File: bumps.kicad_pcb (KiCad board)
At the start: 2 copper layers, 111.1 x 65.4 mm, 135 parts, among them M1 CONN_1, M2 CONN_1, M3 CONN_1, P1 DIL6, P10 Mot-A, P11 Mot-A, P12 Mot-X, P13 T1, P14 T2, P15 T3, P16 MPower, P17 PWM-2, P18 PWM-1, P19 END-X, P2 DIL6, P20 END-Y, P21 END-Z, P22 Mot-X, P23 Mot-Y, P24 Mot-Y, P25 Mot-Z, P26 Mot-Z, P27 Aux, P28 KillSwitch, P29 PWM, P3 Mot-E, P30 CONN_01X01, P31 CONN_01X01, P4 Mot-E, P5 DIL6, P6 DIL6, P7 DIL6, P8 P8 Header, P9 P9 Header, Q1 IRLB8743PBF, Q2 IRLB8743PBF, Q3 FDS9926A, Q4 FDS9926A, U1 Motor-2, U2 Motor-4, U3 Motor-5, U4 Motor-3, U5 Motor-1, U6 MC34063, U7 AP1117/3.3, U8 Opto

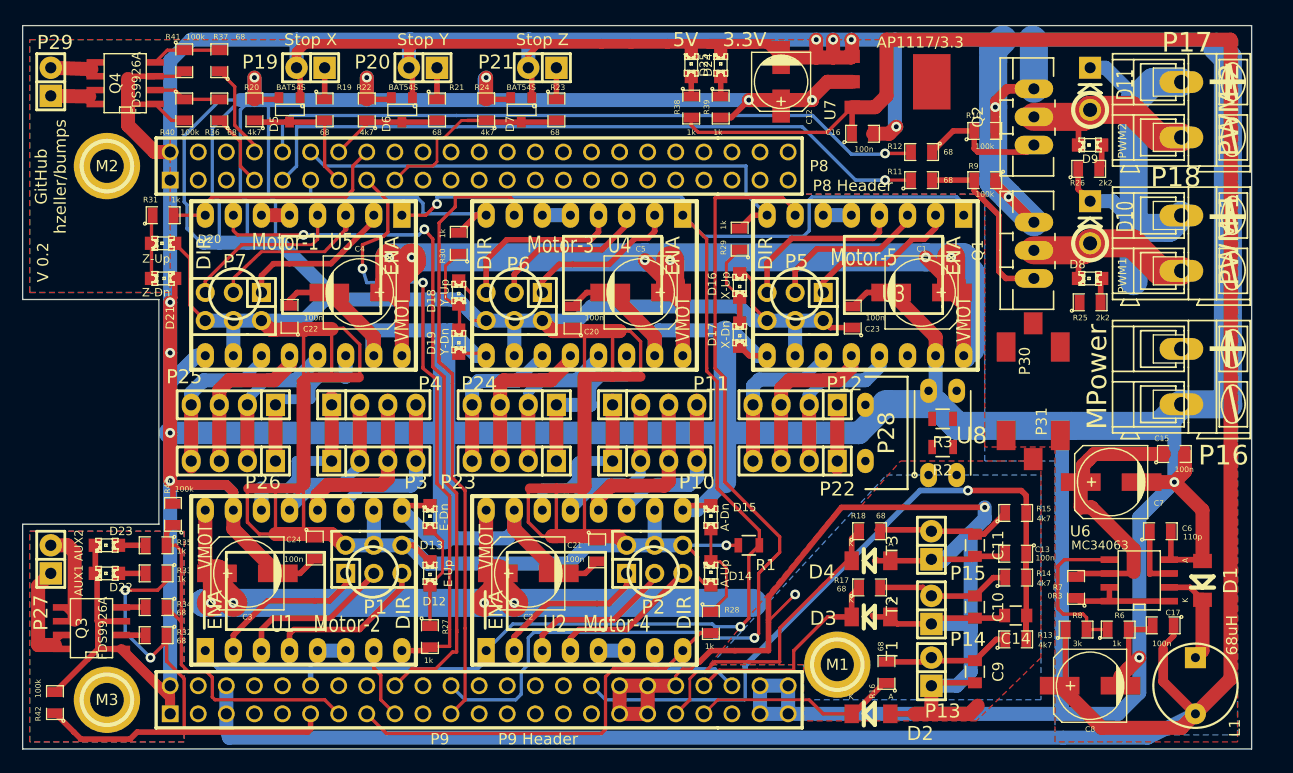
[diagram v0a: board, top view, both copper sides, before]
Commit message: o intermediate state.
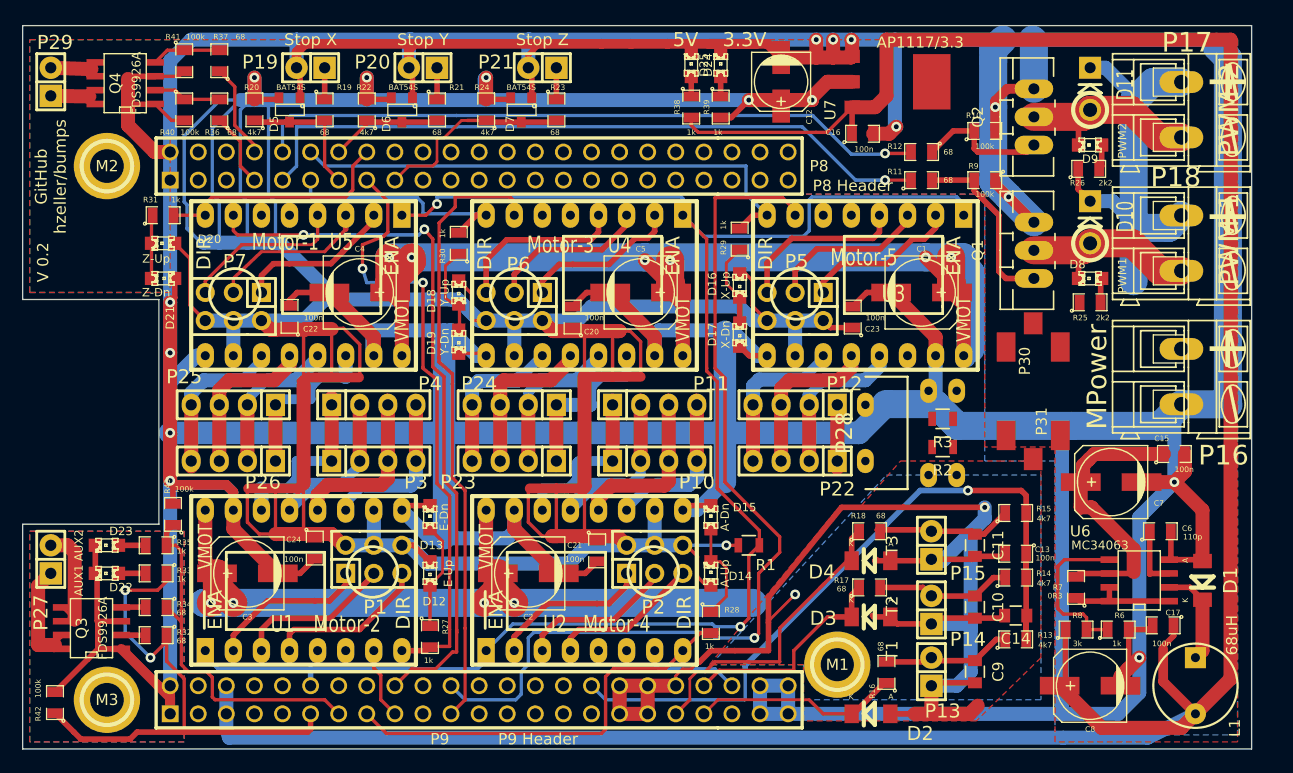
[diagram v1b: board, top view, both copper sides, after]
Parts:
- U8: moved to B.Cu
- turned P28 to 0 degrees
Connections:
- M1 pad 1: Net-(M1-Pad1) -> (no net)
- M2 pad 1: Net-(M2-Pad1) -> (no net)
- M3 pad 1: Net-(M3-Pad1) -> (no net)
- P8 pad 18: Net-(P8-Pad18) -> (no net)
- P8 pad 19: Net-(P8-Pad19) -> (no net)
- P8 pad 20: Net-(P8-Pad20) -> (no net)
- P8 pad 21: Net-(P8-Pad21) -> (no net)
- P8 pad 22: Net-(P8-Pad22) -> (no net)
- P8 pad 23: Net-(P8-Pad23) -> (no net)
- P8 pad 24: Net-(P8-Pad24) -> (no net)
- P8 pad 25: Net-(P8-Pad25) -> (no net)
- P8 pad 26: Net-(P8-Pad26) -> (no net)
- P8 pad 27: Net-(P8-Pad27) -> (no net)
- P8 pad 28: Net-(P8-Pad28) -> (no net)
- P8 pad 29: Net-(P8-Pad29) -> (no net)
- P8 pad 3: Net-(P8-Pad3) -> (no net)
- P8 pad 30: Net-(P8-Pad30) -> (no net)
- P8 pad 31: Net-(P8-Pad31) -> (no net)
- P8 pad 32: Net-(P8-Pad32) -> (no net)
- P8 pad 33: Net-(P8-Pad33) -> (no net)
- P8 pad 34: Net-(P8-Pad34) -> (no net)
- P8 pad 35: Net-(P8-Pad35) -> (no net)
- P8 pad 36: Net-(P8-Pad36) -> (no net)
- P8 pad 37: Net-(P8-Pad37) -> (no net)
- P8 pad 38: Net-(P8-Pad38) -> (no net)
- P8 pad 39: Net-(P8-Pad39) -> (no net)
- P8 pad 4: Net-(P8-Pad4) -> (no net)
- P8 pad 40: Net-(P8-Pad40) -> (no net)
- P8 pad 41: Net-(P8-Pad41) -> (no net)
- P8 pad 42: Net-(P8-Pad42) -> (no net)
- P8 pad 43: Net-(P8-Pad43) -> (no net)
- P8 pad 44: Net-(P8-Pad44) -> (no net)
- P8 pad 45: Net-(P8-Pad45) -> (no net)
- P8 pad 46: Net-(P8-Pad46) -> (no net)
- P8 pad 5: Net-(P8-Pad5) -> (no net)
- P8 pad 6: Net-(P8-Pad6) -> (no net)
- P9 pad 10: Net-(P9-Pad10) -> (no net)
- P9 pad 14: DIR_C -> (no net)
- P9 pad 16: DIR_U -> (no net)
- P9 pad 19: Net-(P9-Pad19) -> (no net)
- P9 pad 20: Net-(P9-Pad20) -> (no net)
- P9 pad 23: DIR_B -> (no net)
- P9 pad 24: STEP_C -> (no net)
- P9 pad 25: Net-(P9-Pad25) -> (no net)
- P9 pad 26: STEP_B -> (no net)
- P9 pad 27: Net-(P9-Pad27) -> (no net)
- P9 pad 28: Net-(P9-Pad28) -> (no net)
- P9 pad 29: Net-(P9-Pad29) -> (no net)
- P9 pad 3: Net-(P9-Pad3) -> (no net)
- P9 pad 30: Net-(P9-Pad30) -> (no net)
- P9 pad 31: Net-(P9-Pad31) -> (no net)
- P9 pad 4: Net-(P9-Pad4) -> (no net)
- P9 pad 41: STEP_U -> (no net)
- P9 pad 7: Net-(P9-Pad7) -> (no net)
- P9 pad 8: Net-(P9-Pad8) -> (no net)
- P9 pad 9: Net-(P9-Pad9) -> (no net)
- U1 pad 5: Net-(U1-Pad5) -> ~EStop
- U1 pad 6: Net-(U1-Pad5) -> (no net)
- U2 pad 5: Net-(U2-Pad5) -> ~EStop
- U2 pad 6: Net-(U2-Pad5) -> (no net)
- U3 pad 5: Net-(U3-Pad5) -> ~EStop
- U3 pad 6: Net-(U3-Pad5) -> (no net)
- U4 pad 5: Net-(U4-Pad5) -> ~EStop
- U4 pad 6: Net-(U4-Pad5) -> (no net)
- U5 pad 5: Net-(U5-Pad5) -> ~EStop
- U5 pad 6: Net-(U5-Pad5) -> (no net)
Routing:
- net Net-(U4-Pad5): track 2.54 -> 0.00 mm
- net Net-(U3-Pad5): track 2.54 -> 0.00 mm
- net Net-(U2-Pad5): track 2.54 -> 0.00 mm
- net Net-(U5-Pad5): track 2.54 -> 0.00 mm
- net Net-(U1-Pad5): track 2.54 -> 0.00 mm
